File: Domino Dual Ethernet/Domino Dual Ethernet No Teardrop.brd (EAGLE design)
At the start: 38.1 x 30.5 mm, 29 parts, among them J1 MH10-1, J2 B50(27-51)FP4-151-A613-B12, J3 B50(27-51)FP4-151-A613-B12, J4 FR04-2, J5 FR04-1

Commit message: Changed copyright
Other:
- board text added: "Reference designs are provided "AS IS" and "WITH ALL FAULTS". The Domino Team disclaims all other warranties express or implied, regarding this product, including but not limited to, any implied warranties of merchantibility or fitness for any particular application."
- board text added: "The Domino Team may make changes to specifications and product descriptions at any time, without notice."
- board text added: "© 2014, The Domino Team. All rights reserved."
- board text removed: "Michel Stempin may make changes to specifications and product descriptions at any time, without notice."
- board text removed: "Reference designs are provided "AS IS" and "WITH ALL FAULTS". Michel Stempin disclaims all other warranties express or implied, regarding this product, including but not limited to, any implied warranties of merchantibility or fitness for any particular application."
- board text removed: "© 2014, Michel Stempin. All rights reserved."
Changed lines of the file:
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@@
 See creativecommons.org/licenses/by-sa/4.0/</text>
 <text x="34.29" y="-51.943" size="0.8128" layer="48" ratio="20">Reference designs are provided "AS IS" and "WITH ALL FAULTS".
-Michel Stempin disclaims all other warranties express or implied,
+The Domino Team disclaims all other warranties express or implied,
 regarding this product, including but not limited to, any implied warranties of
 merchantibility or fitness for any particular application.</text>
-<text x="34.29" y="-55.753" size="0.8128" layer="48" ratio="20">Michel Stempin may make changes to specifications and product descriptions
+<text x="34.29" y="-55.753" size="0.8128" layer="48" ratio="20">The Domino Team may make changes to specifications and product descriptions
 at any time, without notice.</text>
-<text x="74.93" y="-41.91" size="1.27" layer="48" ratio="20">© 2014, Michel Stempin.
+<text x="74.93" y="-41.91" size="1.27" layer="48" ratio="20">© 2014, The Domino Team.
 All rights reserved.</text>
 <text x="115.57" y="-57.15" size="1.778" layer="48">Rev.</text>

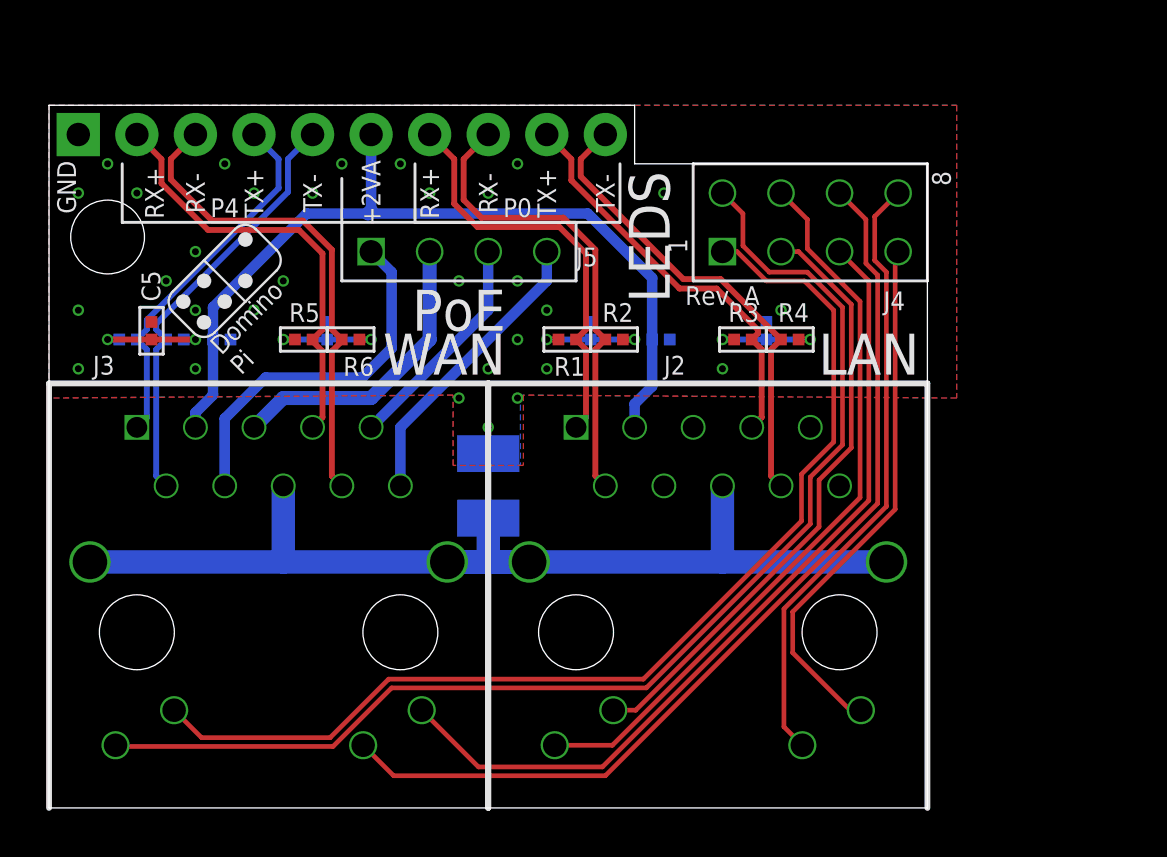
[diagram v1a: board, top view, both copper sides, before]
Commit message: Domino tile Dual Ethernet Revision B
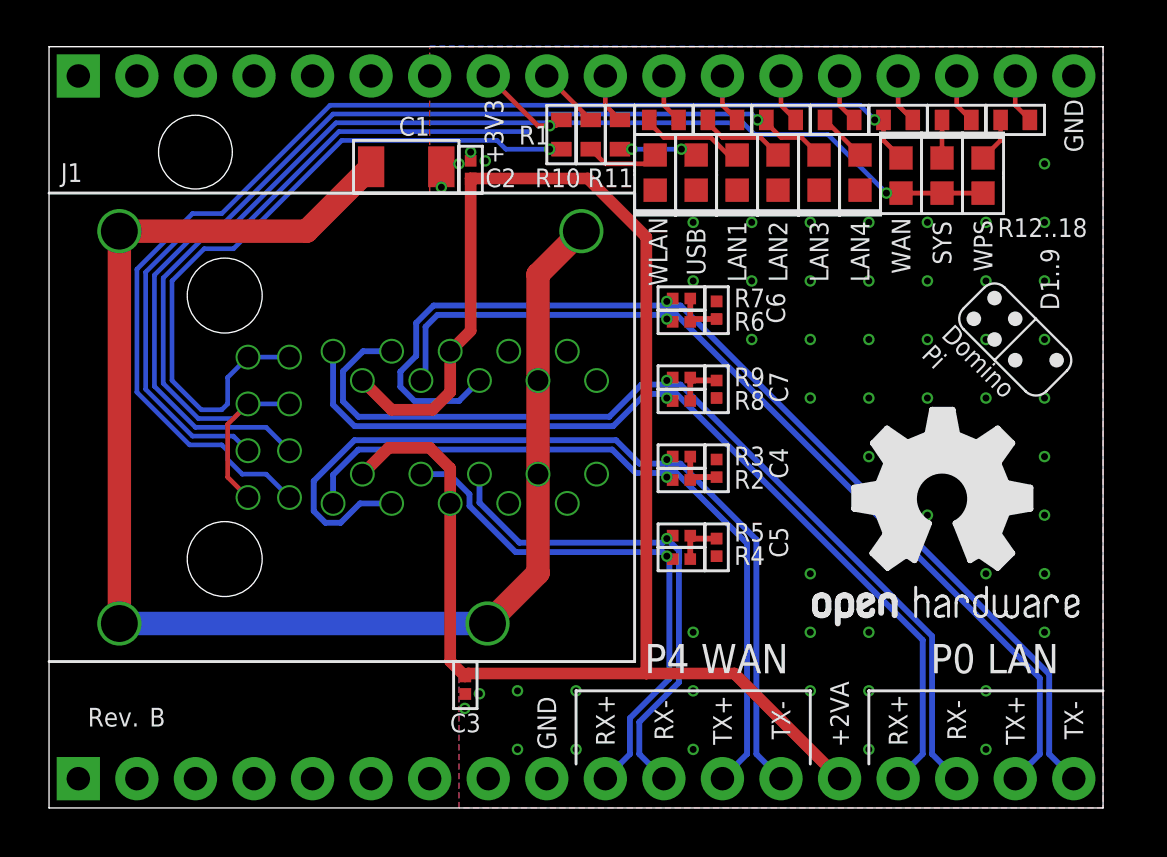
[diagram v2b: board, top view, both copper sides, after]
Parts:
- removed J4: FR04-2, Domino:FR04-2-0.1
- removed J5: FR04-1, Domino:FR04-1-0.1
- added D1: BLUE, Domino:LED0603
- added D2: WHITE, Domino:LED0603
- added D3, D4, D5, D6: GREEN, Domino:LED0603
- added D7: RED, Domino:LED0603
- added D8: ORANGE, Domino:LED0603
- added D9: YELLOW, Domino:LED0603
- added R10, R11, R12, R13, R15: 270R, Domino:R0603
- added R14, R16: 150R, Domino:R0603
- added R17, R18: 330R, Domino:R0603
- added R9: 49R9, Domino:R0402
- added U$13: (no value), Domino:DOMINO_LOGO_SMALL
- added U$16: (no value), Domino:OPEN_HARDWARE_LOGO
- C1: device Domino:C1210 -> Domino:C1206
- J1: value MH10-1 -> B59(57-02)F4-03-1212-C12; device Domino:MH10-1-0.1 -> Domino:B59(57-02)F4-03-1212-C12
- J2, J3: value B50(27-51)FP4-151-A613-B12 -> MH18-1; device Domino:B50(27-51)FP4-151-A613-B12 -> Domino:MH18-1-0.1
- R1: value 49R9 -> 330R; device Domino:R0402 -> Domino:R0603
- moved J2 36.4 mm to (1.27, 31.8), flipped to the bottom, turned to 180 degrees
- moved U$4 32.8 mm to (39.4, 14.6), flipped to the bottom, turned to 270 degrees
- moved C5 26.3 mm to (29.0, 11.3), turned to 90 degrees
- moved R7 24.1 mm to (27.4, 22.1), flipped to the top
- moved R8 22.1 mm to (27.4, 17.7), flipped to the top, turned to 180 degrees
- moved U$7 22.1 mm to (30.5, 12.7)
- moved C6 21.5 mm to (29.0, 21.6), flipped to the top, turned to 270 degrees
- moved U$6 21.0 mm to (9.53, 3.17)
- moved C3 20.2 mm to (18.1, 5.32), flipped to the top, turned to 90 degrees
- moved U$8 19.3 mm to (15.9, 22.2)
- moved R5 18.5 mm to (27.4, 11.8), turned to 180 degrees
- moved C4 17.9 mm to (29.0, 14.7), flipped to the top
- moved U$5 14.5 mm to (17.8, 3.17)
- moved R6 14.4 mm to (27.4, 21.1)
- moved C1 14.3 mm to (15.5, 27.8), flipped to the top, turned to 180 degrees
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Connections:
- removed net P0_LED_L_A: J2.13, J4.8
- removed net P0_LED_L_C: J2.14, J4.7
- removed net P0_LED_R_A: J2.11, J4.4
- removed net P0_LED_R_C: J2.12, J4.3
- removed net P4_LED_L_A: J3.13, J4.6
- removed net P4_LED_L_C: J3.14, J4.5
- removed net P4_LED_R_A: J3.11, J4.2
- removed net P4_LED_R_C: J3.12, J4.1
- removed net VC12: J3.9, J5.3
- removed net VC36: J3.10, J5.4
- removed net VC45: J3.4, J5.1
- removed net VC78: J3.5, J5.2
- new net +3V3: D7.2, D8.2, D9.2, J1.UL2, J2.8, R1.2
- new net LAN1_LED: D3.2, R12.2
- new net LAN2_LED: D4.2, R13.2
- new net LAN3_LED: D5.2, J1.DL2, R14.2
- new net LAN4_LED: D6.2, R15.2
- new net LED0: J2.9, R10.1
- new net LED1: J2.10, R11.1
- new net LED2: J2.11, R12.1
- new net LED3: J2.12, R13.1
- new net LED4: J2.13, R14.1
- new net LED5: J2.14, R15.1
- new net LED6: J2.15, R16.1
- new net LED7: J2.16, R17.1
- new net LED8: J2.17, R18.1
- new net POWER_LED: J1.DL4, J1.UL4, R1.1
- new net SYS_LED: D8.1, R17.2
- new net USB_LED: D2.2, R11.2
- new net WAN_LED: D7.1, J1.UL1, R16.2
- new net WLAN_LED: D1.2, R10.2
- new net WPS_LED: D9.1, R18.2
- net +2VA_ETH_OUT: now also C2.2, C3.2, J1.DR2, J1.DR5, J1.UR2, J1.UR5, J3.14; no longer C6.2, C7.2, J1.6, J2.3, J3.3
- net GND: now also D1.1, D2.1, D3.1, D4.1, D5.1, D6.1, J1.DL1, J1.DL3, J1.UL3, J2.18, J3.9; no longer J1.1
- net P0_RX: now also C7.2, R8.1, R9.1; no longer C2.2, R1.1, R2.1
- net P0_RX_N: now also J1.DR3, J3.16, R9.2; no longer J1.8, J2.2, R2.2
- net P0_RX_P: now also J1.DR1, J3.15, R8.2; no longer J1.7, J2.1, R1.2
- net P0_TX: now also C6.2, R6.1, R7.1; no longer C3.2, R3.1, R4.1
- net P0_TX_N: now also J1.DR6, J3.18, R7.2; no longer J1.10, J2.8, R4.2
- net P0_TX_P: now also J1.DR4, J3.17, R6.2; no longer J1.9, J2.7, R3.2
- net P4_RX: now also C5.2, R4.1; no longer C4.2, R6.1
- net P4_RX_N: now also J1.UR6, J3.11, R5.2; no longer J1.3, J3.8, R6.2
- net P4_RX_P: now also J1.UR4, J3.10, R4.2; no longer J1.2, J3.7, R5.2
- net P4_TX: now also C4.2, R2.1, R3.1; no longer C5.2, R7.1, R8.1
- net P4_TX_N: now also J1.UR3, J3.13, R3.2; no longer J1.5, J3.2, R8.2
- net P4_TX_P: now also J1.UR1, J3.12, R2.2; no longer J1.4, J3.1, R7.2
- net SHIELD: now also J1.DR8, J1.P$1, J1.P$2, J1.P$3, J1.P$4, J1.UR8; no longer J2.6, J2.SH$1, J2.SH$2, J3.6, J3.SH$1, J3.SH$2
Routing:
- net +3V3: track 0.00 -> 56.1 mm, vias 0 -> 2
- net P4_LED_R_A: track 52.3 -> 0.00 mm
- net WAN_LED: track 0.00 -> 51.6 mm, vias 0 -> 1
- net P4_LED_R_C: track 47.2 -> 0.00 mm
- net LAN3_LED: track 0.00 -> 43.5 mm, vias 0 -> 1
- net P4_LED_L_A: track 41.9 -> 0.00 mm
- net P4_LED_L_C: track 36.5 -> 0.00 mm
- net +2VA_ETH_OUT: track 37.7 -> 74.0 mm
- net GND: track 0.00 -> 34.2 mm, vias 31 -> 57
- net P0_LED_R_A: track 32.3 -> 0.00 mm
- net POWER_LED: track 0.00 -> 31.1 mm, vias 0 -> 1
- net P0_LED_L_A: track 26.8 -> 0.00 mm
- net P0_LED_R_C: track 26.4 -> 0.00 mm
- net P0_TX_N: track 20.6 -> 47.0 mm, vias 0 -> 1
- net P0_LED_L_C: track 23.3 -> 0.00 mm
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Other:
- board size 38.1 x 30.5 mm -> 45.7 x 33 mm
- board text added: "+3V3"
- board text added: "7. SILKSCREEN BOARD USING BLACK INK. DISTORTION OF SILKSCREEN IS ACCEPTABLE OVER TRACES. EPOXY INK ON PLATED LANDS IS NOT ACCEPTABLE"
- board text added: "D1..9"
- board text added: "ELD2"
- board text added: "LAN1"
- board text added: "LAN2"
- board text added: "LAN3"
- board text added: "LAN4"
- board text added: "LED0"
- board text added: "LED1"
- board text added: "LED2"
- board text added: "LED3"
- board text added: "LED4"
- board text added: "LED5"
- board text added: "LED6"
- board text added: "LED7"
- board text added: "LED8"
- board text added: "P0 LAN"
- board text added: "P4 WAN"
- board text added: "R12..18"
- board text added: "SYS"
- board text added: "USB"
- board text added: "WLAN"
- board text added: "WPS"
- board text removed: "7. SILKSCREEN BOARD USING WHITE INK. DISTORTION OF SILKSCREEN IS ACCEPTABLE OVER TRACES. EPOXY INK ON PLATED LANDS IS NOT ACCEPTABLE"
- board text removed: "LAN"
- board text removed: "LEDS"
- board text removed: "P0"
- board text removed: "P0_LED_L"
- board text removed: "P0_LED_R"
- board text removed: "P0_RX+"
- board text removed: "P0_RX-"
- board text removed: "P0_TX+"
- board text removed: "P0_TX-"
- board text removed: "P4"
- board text removed: "P4_LED_L"
- board text removed: "P4_LED_R"
- board text removed: "PoE"
- board text removed: "Rev. A"
- board text removed: "VC12"
- board text removed: "VC36"
- board text removed: "VC45"
- board text removed: "VC78"
- board text removed: "_A"
- board text removed: "_C"
